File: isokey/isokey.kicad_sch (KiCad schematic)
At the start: 66 parts, among them J1 PadExp Right, J2 PadExp Left, Q1 BSS138, U1 BlackPill_STLINK, U3 TLV73318PDBV

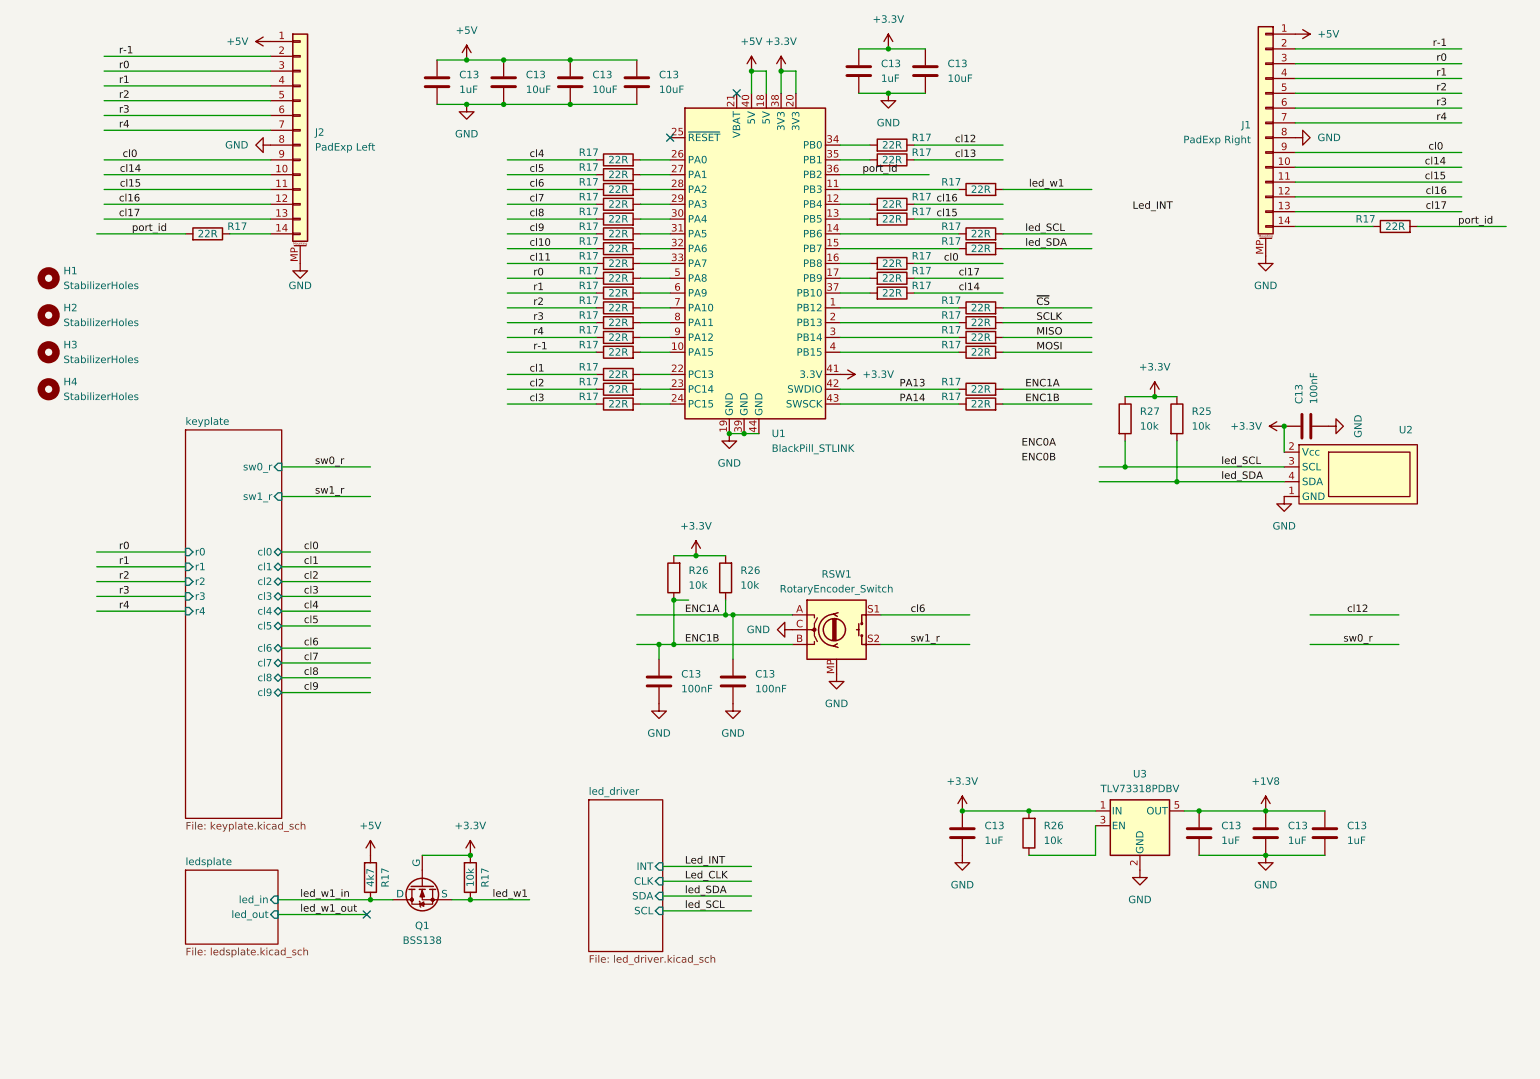
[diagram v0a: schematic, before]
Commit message: Continue routing
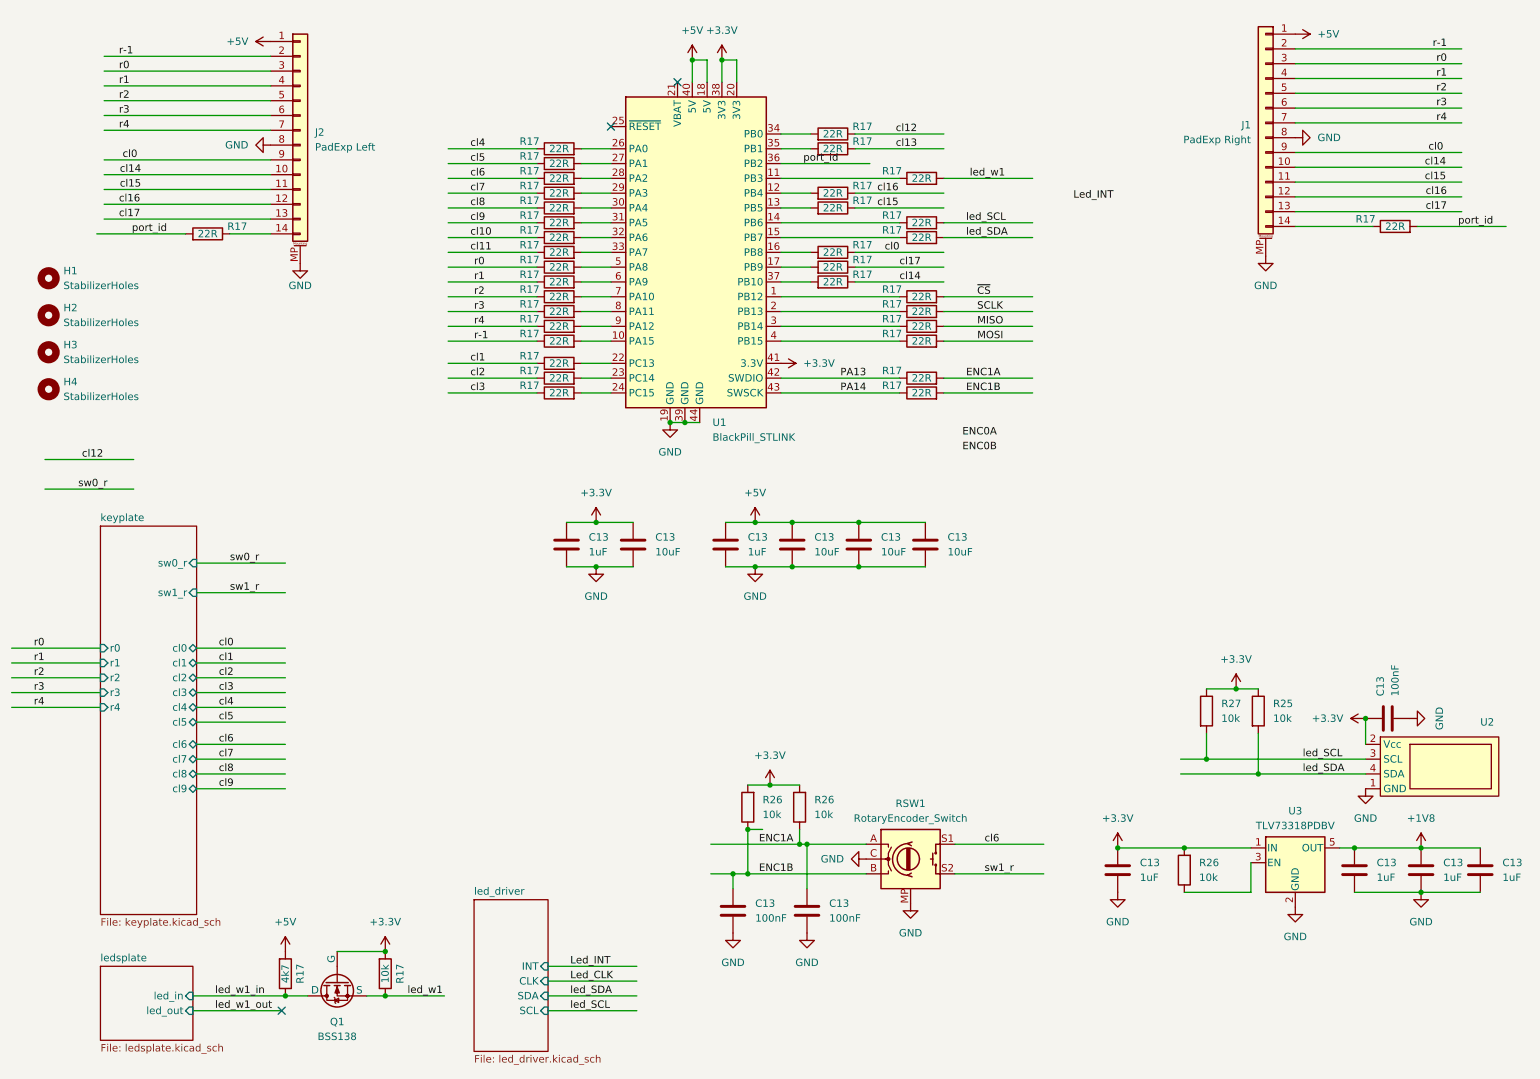
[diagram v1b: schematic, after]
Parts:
- U1: footprint Module:BlackPill -> Module:BlackPill_doble_top-bot
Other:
- moved on the sheet: C13, Q1, R17, R25, R26, R27, RSW1, U1, U2, U3
